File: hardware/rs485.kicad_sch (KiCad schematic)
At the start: 0 parts

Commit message: Almost everything
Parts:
- added U13: MAX3485AEASA+T, EasyEDA:SO-8_L4.9-W3.9-P1.27-LS5.9-BL, symbol EasyEDA:MAX3485AEASA+T
- added U14: KF301-5.0-2P, EasyEDA:CONN-TH_P5.00_KF301-5.0-2P, symbol EasyEDA:KF301-5.0-2P
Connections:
- new net +3V3: U13.8 (VCC)
- new net GND: U13.5 (GND)
- new net RS485_A: U13.6 (A), U14.2
- new net RS485_B: U13.7 (B), U14.1
- new net RS485_MODE: U13.2 (~{RE}), U13.3 (DE)
- new net UART_RX: U13.1 (RO)
- new net UART_TX: U13.4 (DI)

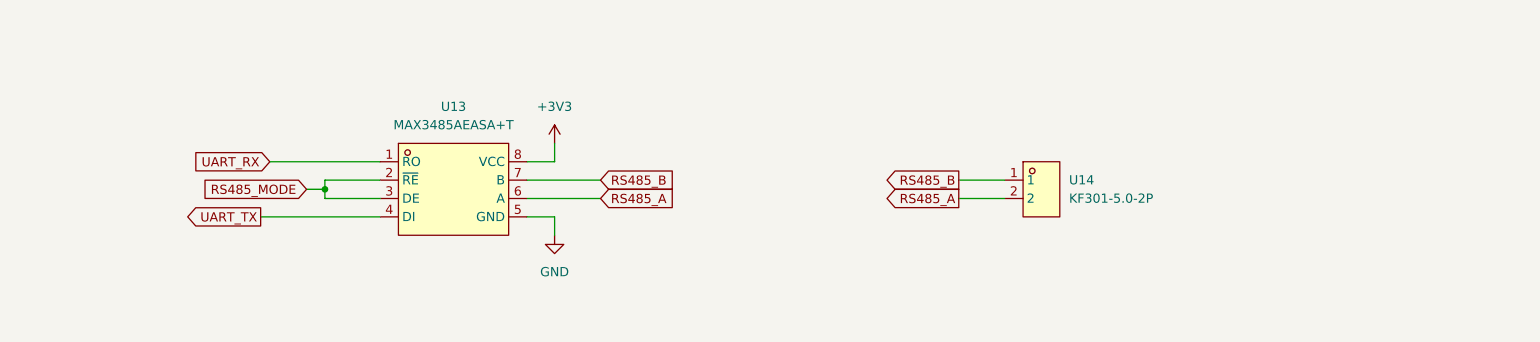
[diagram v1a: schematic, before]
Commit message: Board complete
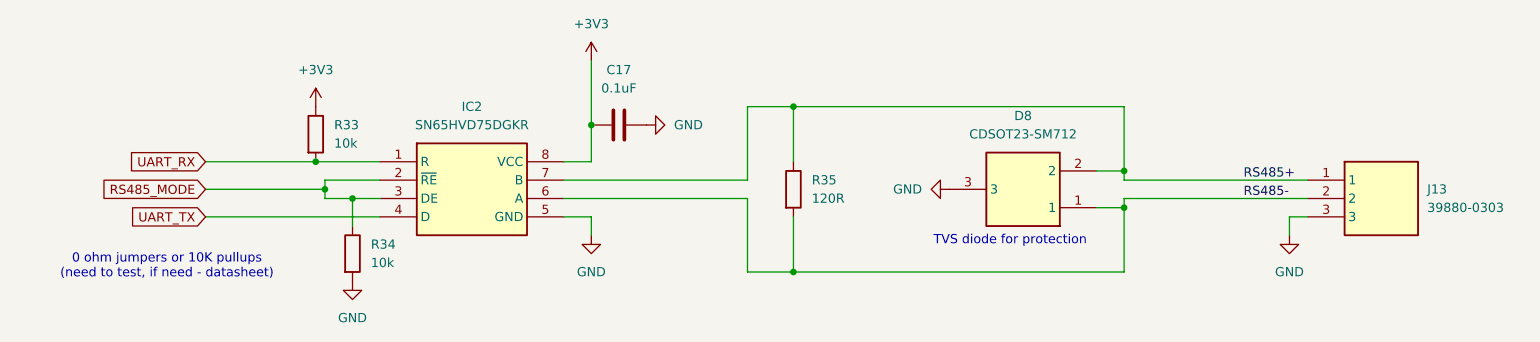
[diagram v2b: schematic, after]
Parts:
- removed U13: MAX3485AEASA+T, EasyEDA:SO-8_L4.9-W3.9-P1.27-LS5.9-BL, symbol EasyEDA:MAX3485AEASA+T
- removed U14: KF301-5.0-2P, EasyEDA:CONN-TH_P5.00_KF301-5.0-2P, symbol EasyEDA:KF301-5.0-2P
- added C17: 0.1uF, Capacitor_SMD:C_1206_3216Metric_Pad1.33x1.80mm_HandSolder, symbol Device:C
- added D8: CDSOT23-SM712, Samacsys:SOT95P230X117-3N, symbol Samacsys:CDSOT23-SM712
- added IC2: SN65HVD75DGKR, Samacsys:SOP65P490X110-8N, symbol Samacsys:SN65HVD75DGKR
- added J13: 39880-0303, Samacsys:398800303, symbol Samacsys:39880-0303
- added R33, R34: 10k, Resistor_SMD:R_1206_3216Metric_Pad1.30x1.75mm_HandSolder, symbol Device:R
- added R35: 120R, Resistor_SMD:R_1206_3216Metric_Pad1.30x1.75mm_HandSolder, symbol Device:R
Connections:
- net +3V3: now also C17.1, IC2.8 (VCC), R33.1
- net GND: now also C17.2, D8.3, IC2.5 (GND), J13.3, R34.2
- net RS485_MODE: now also IC2.2 (~{RE}), IC2.3 (DE), R34.1
- net UART_RX: now also IC2.1 (R), R33.2
- net UART_TX: now also IC2.4 (D)
- new net RS485+: D8.2, IC2.7 (B), J13.1, R35.1
- new net RS485-: D8.1, IC2.6 (A), J13.2, R35.2
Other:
- note added: "0 ohm jumpers or 10K pullups (need to test, if need - datasheet)"
- note added: "TVS diode for protection"
